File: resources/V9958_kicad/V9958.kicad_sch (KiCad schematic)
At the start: 47 parts, among them U1 NMOS, U10 NMOS, U11 NMOS, U12 NMOS, U13 NMOS, U16 AND2, U17 DSR, U18 NOR6, U19 DSR, U2 NOR2, U20 DSR, U21 DSR, U22 DSR, U23 DSR, U24 DSR, U25 DSR, U26 BUF, U27 INVP, U28 NOR2, U29 NOR2, U3 INV, U30 DSR, U31 DSR, U32 DSR, U35 NOR4, U36 DSR, U37 DSR, U38 DSR, U39 NOR2, U4 INV, U40 BUFP, U41 DSR, U42 INV, U43 BUFP, U44 NMOS, U45 NMOS, U46 NOR2, U47 NOR2, U48 INV, U49 INV, U5 INV, U50 NOR2, U51 NOR2, U6 NMOS, U7 NMOS, U8 NMOS, U9 NOR2

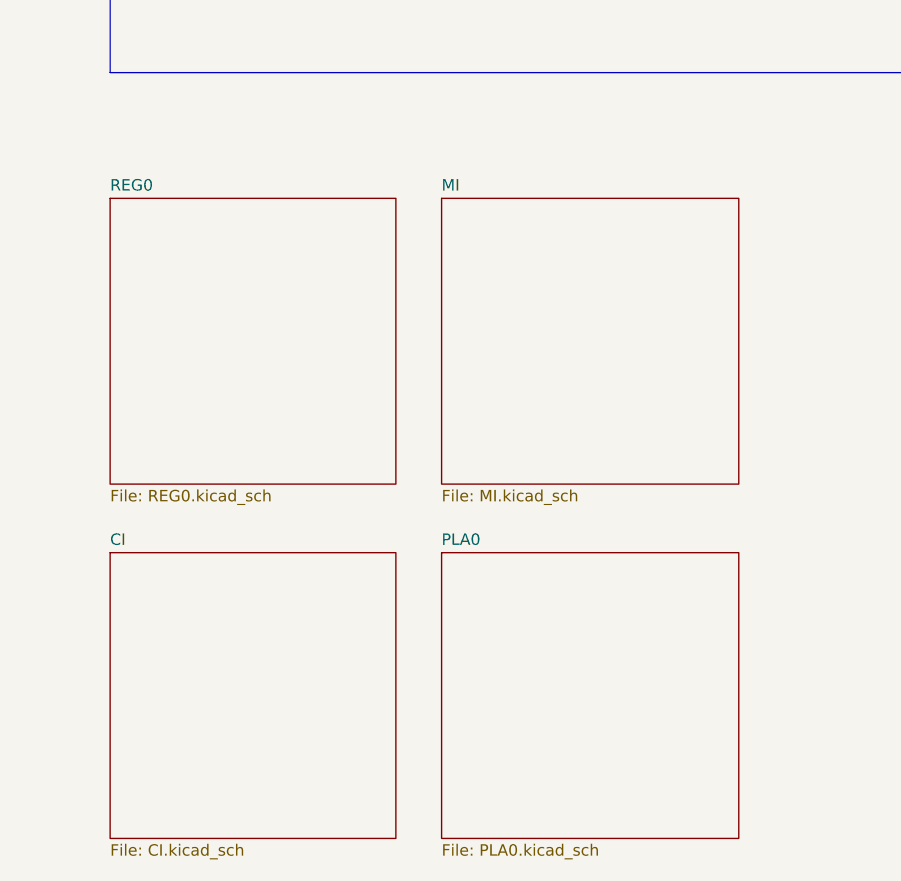
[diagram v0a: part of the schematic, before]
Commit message: update 20250809
HVCNTR
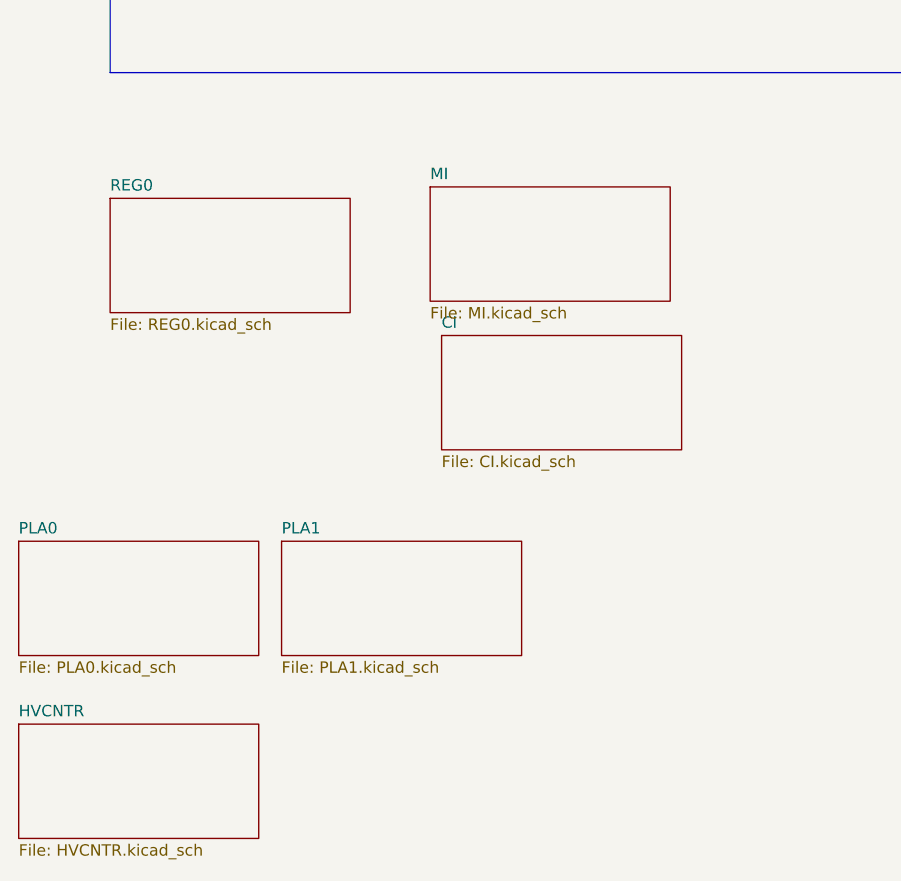
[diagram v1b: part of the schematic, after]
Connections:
- net at U18.: now also U24. (Φ2); no longer U17. (Φ2)
- net at U43.: now also U44.; no longer U42.
- net at U48.: now also U21. (Φ2), U46.; no longer U47.
- net at U40.: now also U45.; no longer U39.
- net at U27.: now also U16.; no longer U25. (Φ2)
- new net: U18., U19. (Φ2), U20. (Φ2), U29.
- new net: U18., U20. (Φ2), U28.
- new net: U17. (Φ2), U18., U19. (Φ2), U28., U29.
- new net: U17. (Φ2), U18.
- new net: U18., U36. (Φ2)
- new net: U18., U23. (Φ2), U24. (Φ2)
- new net: U1., U2., U8.
- new net: U1., U6., U7.
- new net: U42., U43.
- new net: U47., U48.
- new net: U38. (Φ2), U39.
- new net: U39., U40.
- new net: U31. (Φ2), U32. (Φ2), U35.
- new net: U32. (Φ2), U35.
- new net: U10., U11., U13.
- new net: U37. (Φ2), U49., U50.
- new net: U22. (Φ2), U23. (Φ2)
- new net: U16., U22. (Φ2)
- new net: U11., U12., U9.
- new net: U28., U37. (Φ2), U41. (Φ2)
- new net: U21. (Φ2), U29., U30. (Φ2), U38. (Φ2)
- new net: U25. (Φ2), U27.
- new net: U25. (Φ2), U26.
- new net: U10., U5., U9.
- new net: U2., U3., U6.
- new net: U30. (Φ2), U31. (Φ2)
- new net: U35., U36. (Φ2)
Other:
- added sheet HVCNTR (HVCNTR.kicad_sch)
- added sheet PLA1 (PLA1.kicad_sch)
